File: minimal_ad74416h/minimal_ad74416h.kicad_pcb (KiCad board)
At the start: 4 copper layers, 30.5 x 25.4 mm, 37 parts, among them U1 AD74416HBCPZ-RL7

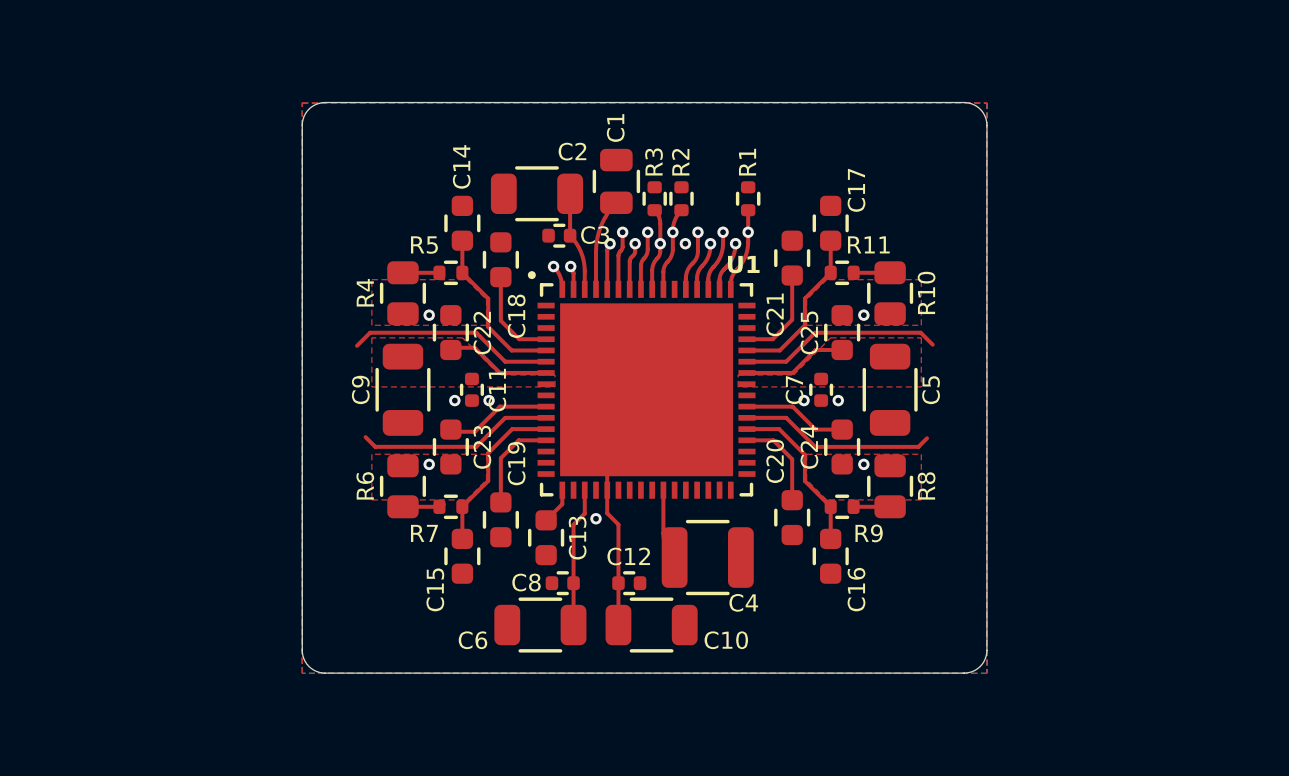
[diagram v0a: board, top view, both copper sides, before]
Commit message: backup
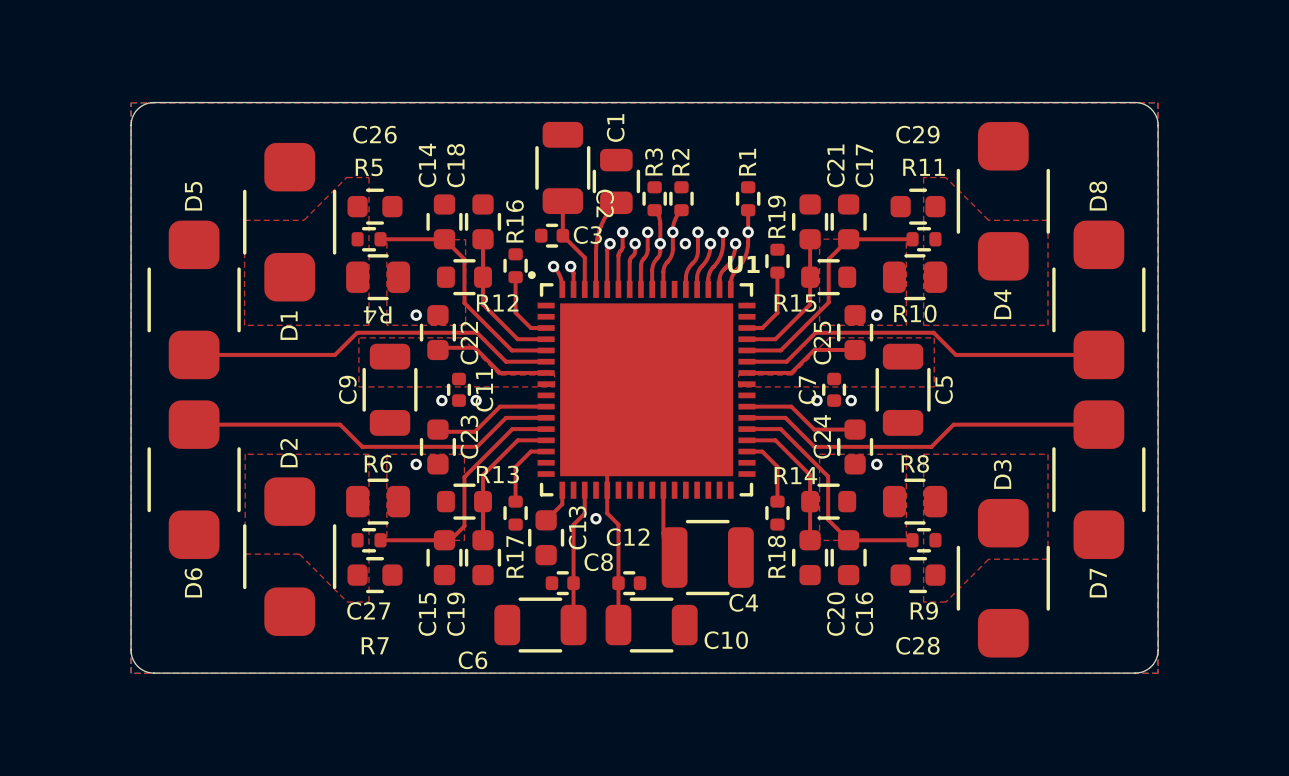
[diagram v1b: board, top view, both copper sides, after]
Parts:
- added C26: 4.7 nF, capacitor_footprints:C_0603_1608Metric, F.Cu at (123.4, 105.3)
- added C27: 4.7 nF, capacitor_footprints:C_0603_1608Metric, F.Cu at (123.4, 121.7)
- added C28: 4.7 nF, capacitor_footprints:C_0603_1608Metric, F.Cu at (147.6, 121.7)
- added C29: 4.7 nF, capacitor_footprints:C_0603_1608Metric, F.Cu at (147.6, 105.3)
- added D1: 36 V, diode_footprints:DO-214AA, F.Cu at (119.6, 105.9)
- added D2: 36 V, diode_footprints:DO-214AA, F.Cu at (119.6, 120.8)
- added D3: 36 V, diode_footprints:DO-214AA, F.Cu at (151.4, 121.8)
- added D4: 36 V, diode_footprints:DO-214AA, F.Cu at (151.4, 105.0)
- added D5: 36 V, diode_footprints:DO-214AA, F.Cu at (115.3, 109.4)
- added D6: 36 V, diode_footprints:DO-214AA, F.Cu at (115.3, 117.4)
- added D7: 36 V, diode_footprints:DO-214AA, F.Cu at (155.6, 117.4)
- added D8: 36 V, diode_footprints:DO-214AA, F.Cu at (155.6, 109.4)
- added R12: 2 kΩ, resistor_footprints:R_0603_1608Metric, F.Cu at (127.4, 108.4)
- added R13: 2 kΩ, resistor_footprints:R_0603_1608Metric, F.Cu at (127.4, 118.4)
- added R14: 2 kΩ, resistor_footprints:R_0603_1608Metric, F.Cu at (143.6, 118.4)
- added R15: 2 kΩ, resistor_footprints:R_0603_1608Metric, F.Cu at (143.6, 108.4)
- added R16: 2 kΩ, resistor_footprints:R_0402_1005Metric, F.Cu at (129.6, 107.9)
- added R17: 2 kΩ, resistor_footprints:R_0402_1005Metric, F.Cu at (129.6, 118.9)
- added R18: 2 kΩ, resistor_footprints:R_0402_1005Metric, F.Cu at (141.3, 118.9)
- added R19: 2 kΩ, resistor_footprints:R_0402_1005Metric, F.Cu at (141.3, 107.7)
- moved R11 3.94 mm to (147.8, 106.7)
- moved R5 3.94 mm to (123.1, 106.7)
- moved R9 3.94 mm to (147.8, 120.1)
- moved R7 3.94 mm to (123.1, 120.1)
- moved C20 1.96 mm to (142.8, 120.9)
- moved C18 1.87 mm to (128.2, 105.9)
- moved C19 1.86 mm to (128.2, 120.9)
- moved C21 1.80 mm to (142.8, 105.9)
- moved C2 1.63 mm to (131.7, 103.5), turned to 90 degrees
- moved R4 1.32 mm to (123.5, 108.4), turned to 180 degrees
- moved R10 1.32 mm to (147.4, 108.4), turned to 0 degrees
- moved R6 1.30 mm to (123.5, 118.4), turned to 180 degrees
- moved R8 1.30 mm to (147.4, 118.4), turned to 0 degrees
- moved C17 0.80 mm to (144.5, 105.9)
- moved C16 0.80 mm to (144.5, 120.9)
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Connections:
- net Net-(R10-Pad2) renamed /I/OP_D
- net Net-(R4-Pad2) renamed /I/OP_A
- net Net-(R6-Pad2) renamed /I/OP_B
- net Net-(R8-Pad2) renamed /I/OP_C
- U1 pad 11: unconnected-(U1-VSENSEN_B-Pad11) -> /VSENSEN_B
- U1 pad 14: unconnected-(U1-VSENSEP_B-Pad14) -> /VSENSEP_B
- U1 pad 3: unconnected-(U1-VSENSEP_A-Pad3) -> /VSENSEP_A
- U1 pad 35: unconnected-(U1-VSENSEP_C-Pad35) -> /VSENSEP_C
- U1 pad 38: unconnected-(U1-VSENSEN_C-Pad38) -> /VSENSEN_C
- U1 pad 43: unconnected-(U1-VSENSEN_D-Pad43) -> /VSENSEN_D
- U1 pad 46: unconnected-(U1-VSENSEP_D-Pad46) -> /VSENSEP_D
- U1 pad 6: unconnected-(U1-VSENSEN_A-Pad6) -> /VSENSEN_A
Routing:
- net /VSENSEN_A: track 0.00 -> 16.6 mm
- net /VSENSEN_B: track 0.00 -> 16.6 mm
- net /VSENSEN_C: track 0.00 -> 16.6 mm
- net /VSENSEN_D: track 0.00 -> 16.6 mm
- net unconnected-(U1-VSENSEN_A-Pad6): track 9.19 -> 0.00 mm
- net unconnected-(U1-VSENSEN_D-Pad43): track 9.02 -> 0.00 mm
- net unconnected-(U1-VSENSEN_B-Pad11): track 8.75 -> 0.00 mm
- net unconnected-(U1-VSENSEN_C-Pad38): track 8.71 -> 0.00 mm
- net /VSENSEP_D: track 0.00 -> 3.43 mm
- net /SENSELF_C: track 7.27 -> 10.5 mm
- net /SENSELF_D: track 7.29 -> 10.6 mm
- net /SENSELF_A: track 7.33 -> 10.6 mm
- net /VSENSEP_A: track 0.00 -> 3.22 mm
- net /VSENSEP_C: track 0.00 -> 3.19 mm
- net /VSENSEP_B: track 0.00 -> 3.19 mm
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- added copper zone on F.Cu, net /I/OP_A
- added copper zone on F.Cu, net /I/OP_B
- added copper zone on F.Cu, net /I/OP_C
- added copper zone on F.Cu, net /I/OP_D
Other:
- board size 30.5 x 25.4 mm -> 45.7 x 25.4 mm

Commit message: backup
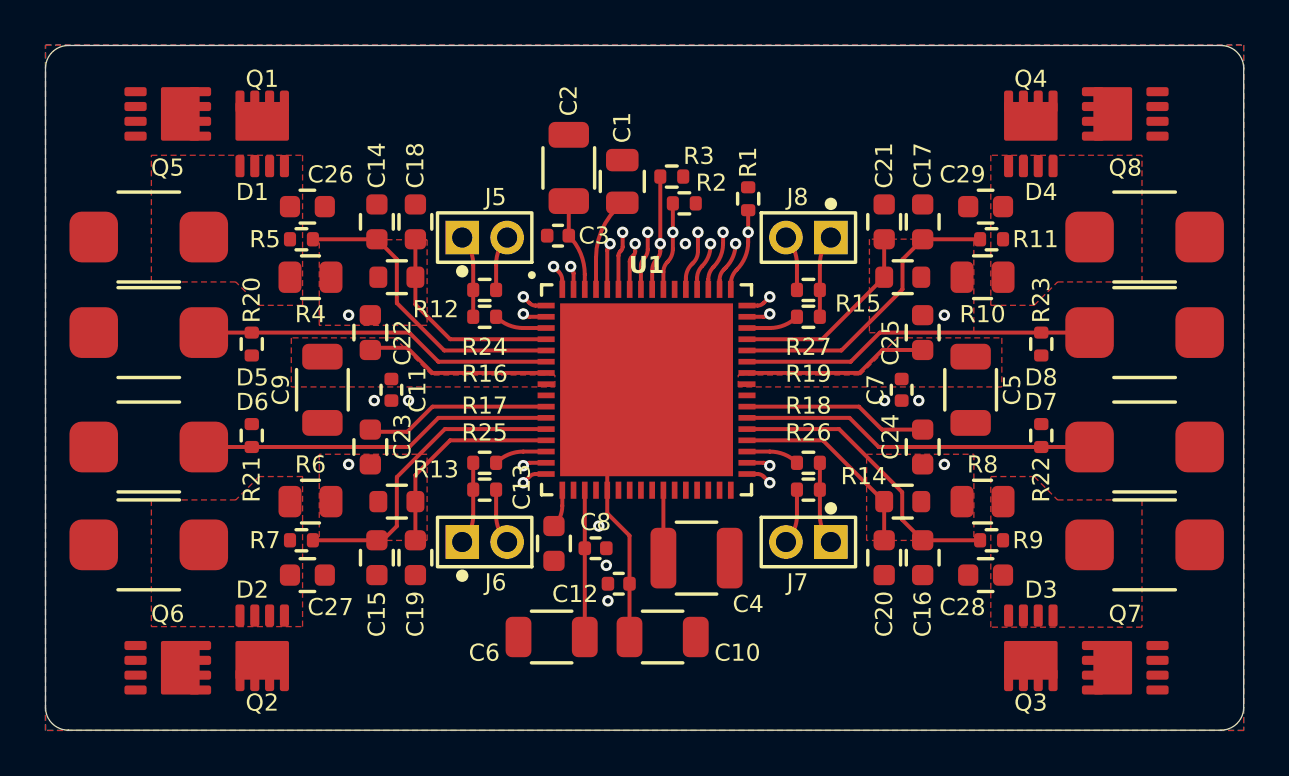
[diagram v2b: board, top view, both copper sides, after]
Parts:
- added J5: MTMM-101-04-L-D-196, connector_footprints:MTMM-101-04-L-D-196, F.Cu at (128.3, 106.6)
- added J6: MTMM-101-04-L-D-196, connector_footprints:MTMM-101-04-L-D-196, F.Cu at (128.3, 120.2)
- added J7: MTMM-101-04-L-D-196, connector_footprints:MTMM-101-04-L-D-196, F.Cu at (142.7, 120.2)
- added J8: MTMM-101-04-L-D-196, connector_footprints:MTMM-101-04-L-D-196, F.Cu at (142.7, 106.6)
- added Q1: -100.0 V, transistor_footprints:PowerPAK 1212-8, F.Cu at (118.4, 102.0)
- added Q2: -100.0 V, transistor_footprints:PowerPAK 1212-8, F.Cu at (118.4, 124.9)
- added Q3: -100.0 V, transistor_footprints:PowerPAK 1212-8, F.Cu at (152.6, 124.9)
- added Q4: -100.0 V, transistor_footprints:PowerPAK 1212-8, F.Cu at (152.6, 102.0)
- added Q5: -100.0 V, transistor_footprints:PowerPAK 1212-8, F.Cu at (114.2, 101.1)
- added Q6: -100.0 V, transistor_footprints:PowerPAK 1212-8, F.Cu at (114.2, 125.8)
- added Q7: -100.0 V, transistor_footprints:PowerPAK 1212-8, F.Cu at (156.8, 125.8)
- added Q8: -100.0 V, transistor_footprints:PowerPAK 1212-8, F.Cu at (156.8, 101.1)
- added R20: 100 kΩ, resistor_footprints:R_0402_1005Metric, F.Cu at (117.9, 111.4)
- added R21: 100 kΩ, resistor_footprints:R_0402_1005Metric, F.Cu at (117.9, 115.4)
- added R22: 100 kΩ, resistor_footprints:R_0402_1005Metric, F.Cu at (153.0, 115.4)
- added R23: 100 kΩ, resistor_footprints:R_0402_1005Metric, F.Cu at (153.0, 111.4)
- added R24: 10 kΩ, resistor_footprints:R_0402_1005Metric, F.Cu at (128.3, 109.0)
- added R25: 10 kΩ, resistor_footprints:R_0402_1005Metric, F.Cu at (128.3, 117.9)
- added R26: 10 kΩ, resistor_footprints:R_0402_1005Metric, F.Cu at (142.7, 117.9)
- added R27: 10 kΩ, resistor_footprints:R_0402_1005Metric, F.Cu at (142.7, 109.0)
- moved D4 6.49 mm to (157.6, 106.6), turned to 180 degrees
- moved D3 6.46 mm to (157.6, 120.3), turned to 180 degrees
- moved D1 6.31 mm to (113.3, 106.6), turned to 0 degrees
- moved D2 6.30 mm to (113.3, 120.3), turned to 0 degrees
- moved C16 3.30 mm to (147.8, 120.9)
- moved C17 3.30 mm to (147.8, 105.9)
- moved C20 3.30 mm to (146.0, 120.9)
- moved C21 3.30 mm to (146.0, 105.9)
- moved R14 3.30 mm to (146.9, 118.4)
- moved R15 3.30 mm to (146.9, 108.4)
- moved C11 3.01 mm to (124.1, 113.4)
- moved C14 3.01 mm to (123.5, 105.9)
- moved C15 3.01 mm to (123.5, 120.9)
- moved C26 3.01 mm to (120.4, 105.3)
- moved C27 3.01 mm to (120.4, 121.7)
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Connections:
- net /VSENSEN_A renamed /ISN_A
- net /VSENSEN_B renamed /ISN_B
- net /VSENSEN_C renamed /ISN_C
- net /VSENSEN_D renamed /ISN_D
- R16 pad 2: unconnected-(R16-Pad2) -> /ISP_A
- R17 pad 2: unconnected-(R17-Pad2) -> /ISP_B
- R18 pad 2: unconnected-(R18-Pad2) -> /ISP_C
- R19 pad 2: unconnected-(R19-Pad2) -> /ISP_D
- U1 pad 15: unconnected-(U1-LKG_COMP_B-Pad15) -> /LKG_COMP_B
- U1 pad 2: unconnected-(U1-LKG_COMP_A-Pad2) -> /LKG_COMP_A
- U1 pad 34: unconnected-(U1-LKG_COMP_C-Pad34) -> /LKG_COMP_C
- U1 pad 47: unconnected-(U1-LKG_COMP_D-Pad47) -> /LKG_COMP_D
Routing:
- net /ISP_B: track 0.00 -> 3.65 mm
- net /ISP_D: track 0.00 -> 3.65 mm
- net /ISP_C: track 0.00 -> 3.65 mm
- net /ISP_A: track 0.00 -> 3.65 mm
- net /SENSELF_B: track 10.2 -> 13.2 mm
- net /SENSELF_A: track 10.6 -> 13.6 mm
- net /SENSEHF_A: track 6.35 -> 9.36 mm
- net /SENSEHF_B: track 6.35 -> 9.36 mm
- net /CCOMP_B: track 5.28 -> 8.29 mm
- net /CCOMP_A: track 5.28 -> 8.29 mm
- net /CCOMP_C: track 5.24 -> 8.24 mm
- net /CCOMP_D: track 5.24 -> 8.24 mm
- net /SENSELF_D: track 10.6 -> 13.5 mm
- net /SENSEHF_C: track 6.36 -> 8.96 mm
- net /SENSELF_C: track 10.5 -> 13.1 mm
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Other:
- board size 45.7 x 25.4 mm -> 53.3 x 30.5 mm
